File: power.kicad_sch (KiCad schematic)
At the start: 38 parts, among them U5 TI LMR54410DBV, U6 TI LMR54410DBV, U7 TI TPS2553DBVR-1, U8 TI TPS2553DBVR-1

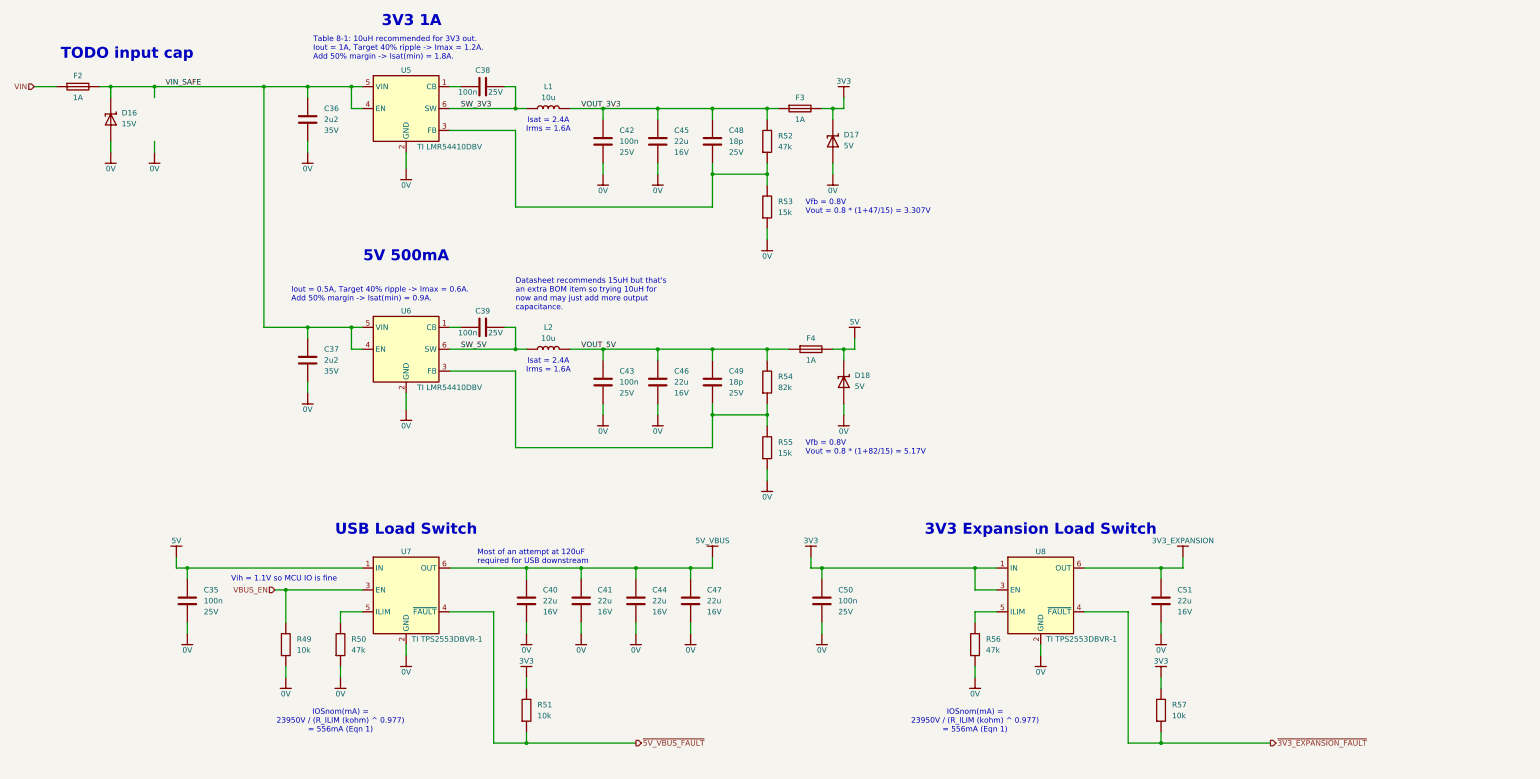
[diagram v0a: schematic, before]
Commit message: draft v1 release
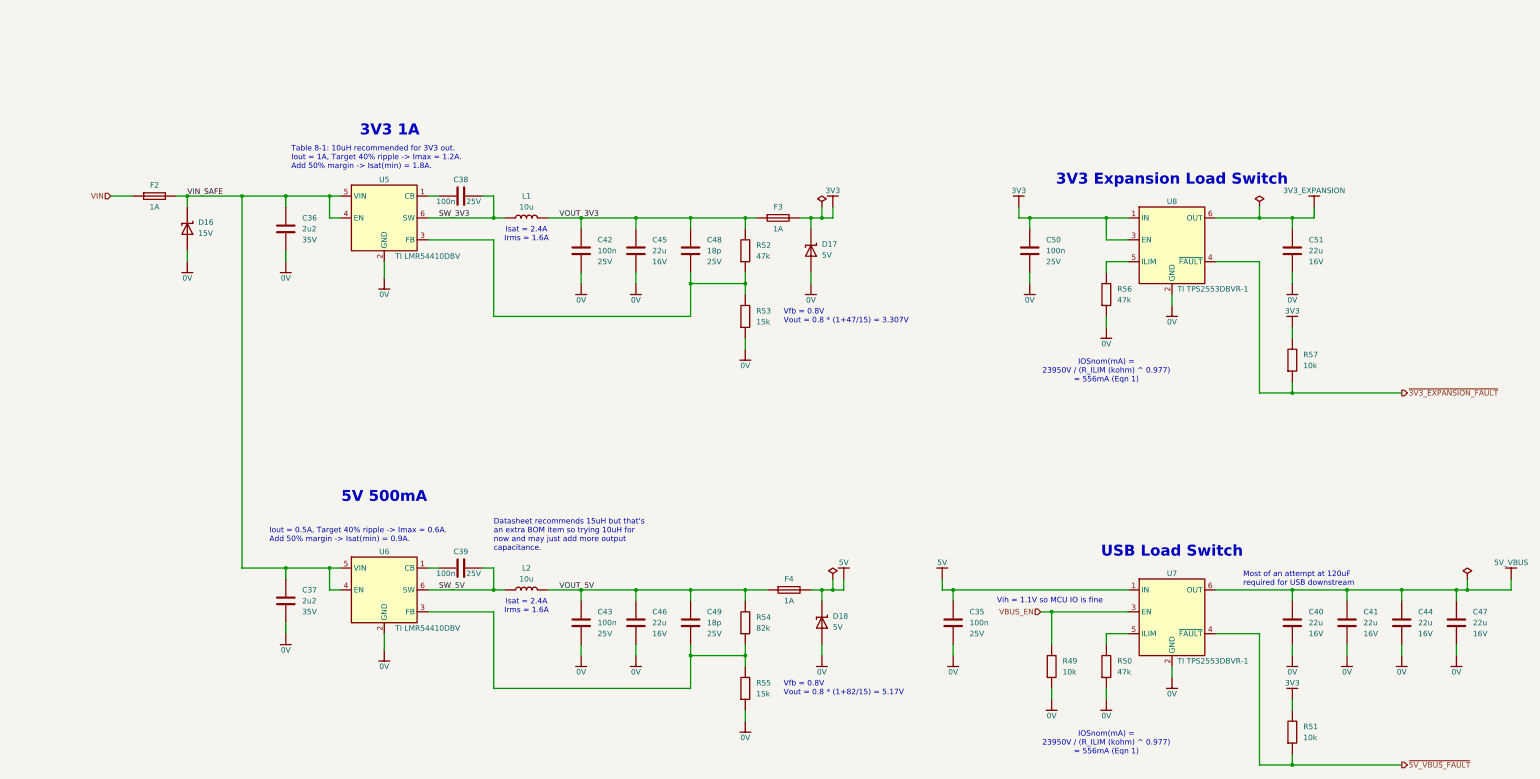
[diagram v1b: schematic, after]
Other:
- note removed: "TODO input cap"
- moved on the sheet: C35, C36, C37, C38, C39, C40, C41, C42, C43, C44, C45, C46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
